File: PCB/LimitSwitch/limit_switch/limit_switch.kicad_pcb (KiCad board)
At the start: 2 copper layers, 40.6 x 38.1 mm, 30 parts, among them J2 Conn_01x06, J3 Conn_01x08, J4 Conn_01x08, J5 Conn_01x08, J6 Conn_01x08, U1 PC817, U2 PC817, U3 PC817, U4 PC817

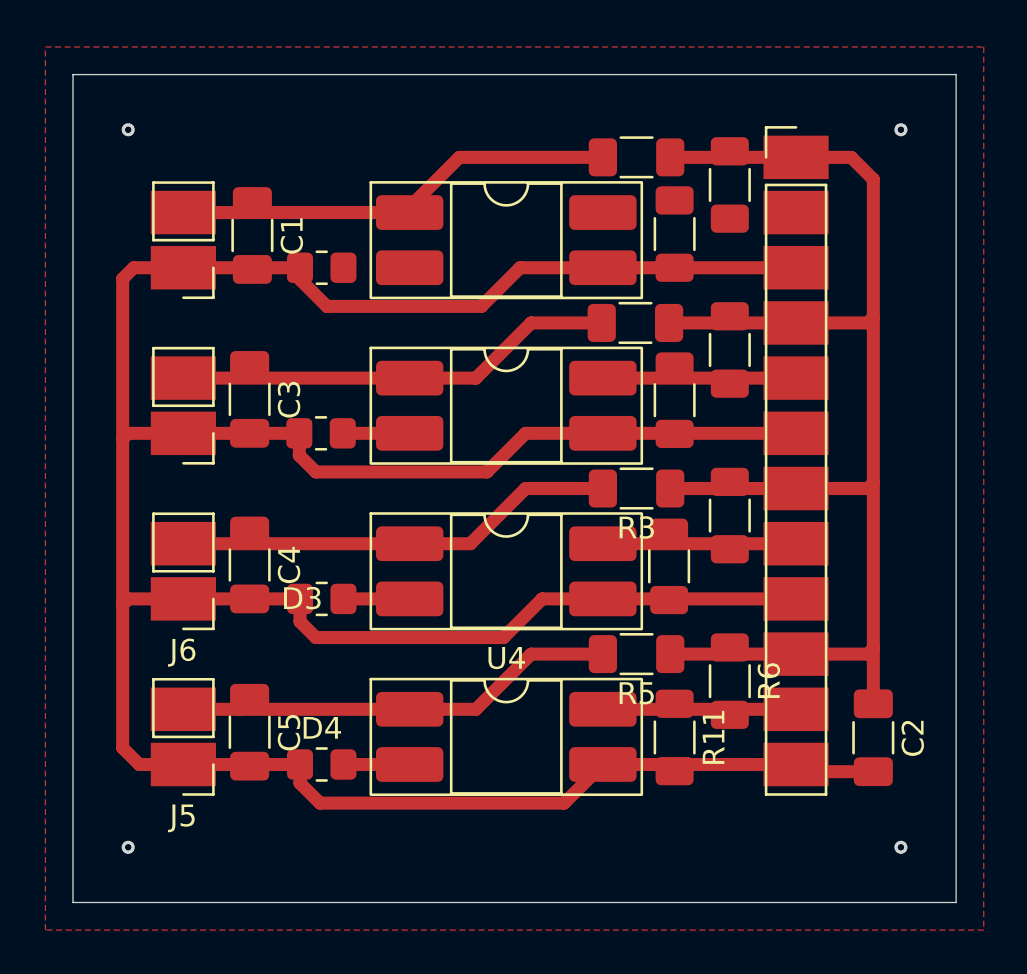
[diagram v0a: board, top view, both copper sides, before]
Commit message: 3
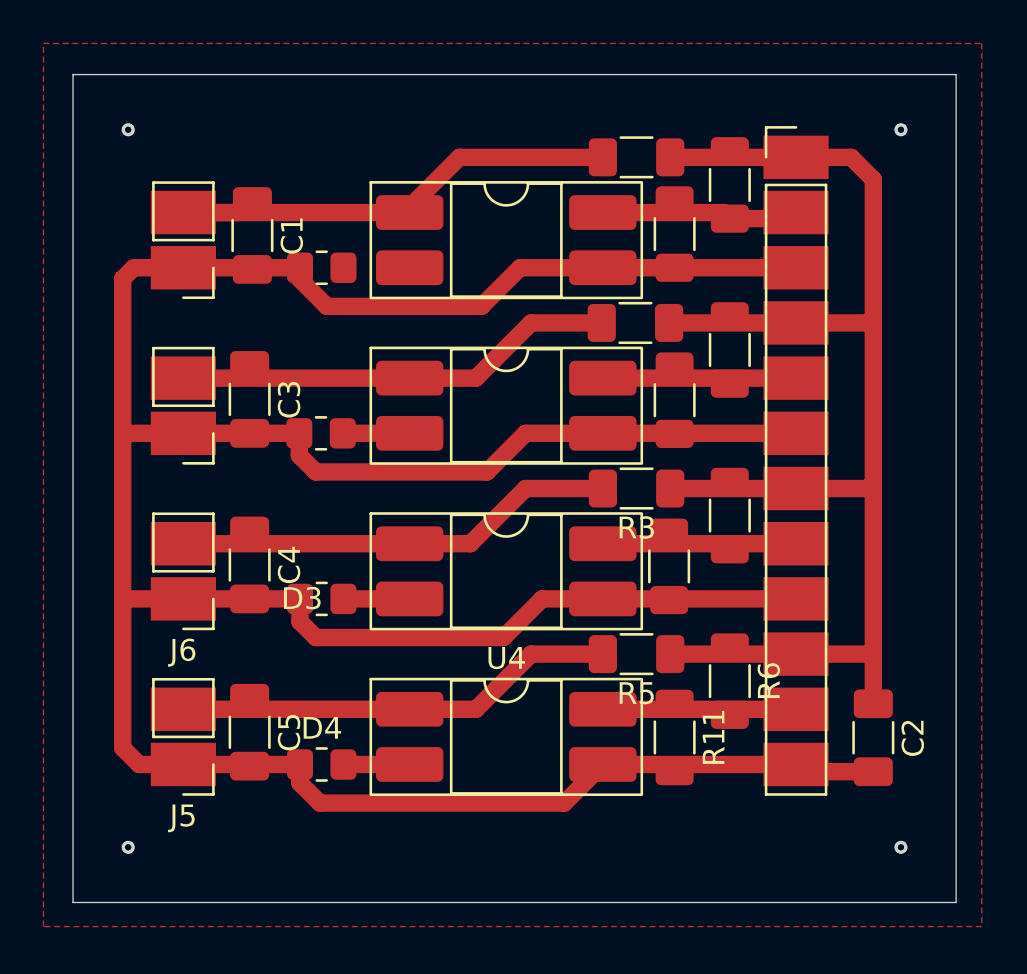
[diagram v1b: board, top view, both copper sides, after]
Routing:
- net PIN1_OUT: track 0.00 -> 9.12 mm
